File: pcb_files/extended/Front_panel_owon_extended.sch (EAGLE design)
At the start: 17 parts, among them M1 ARDUINO-NANO-3.0, SW1 ROTARTY_ENCODER, SW2 TACTILE-SWITCH-PTH, SW3 TACTILE-SWITCH-PTH, SW4 TACTILE-SWITCH-PTH

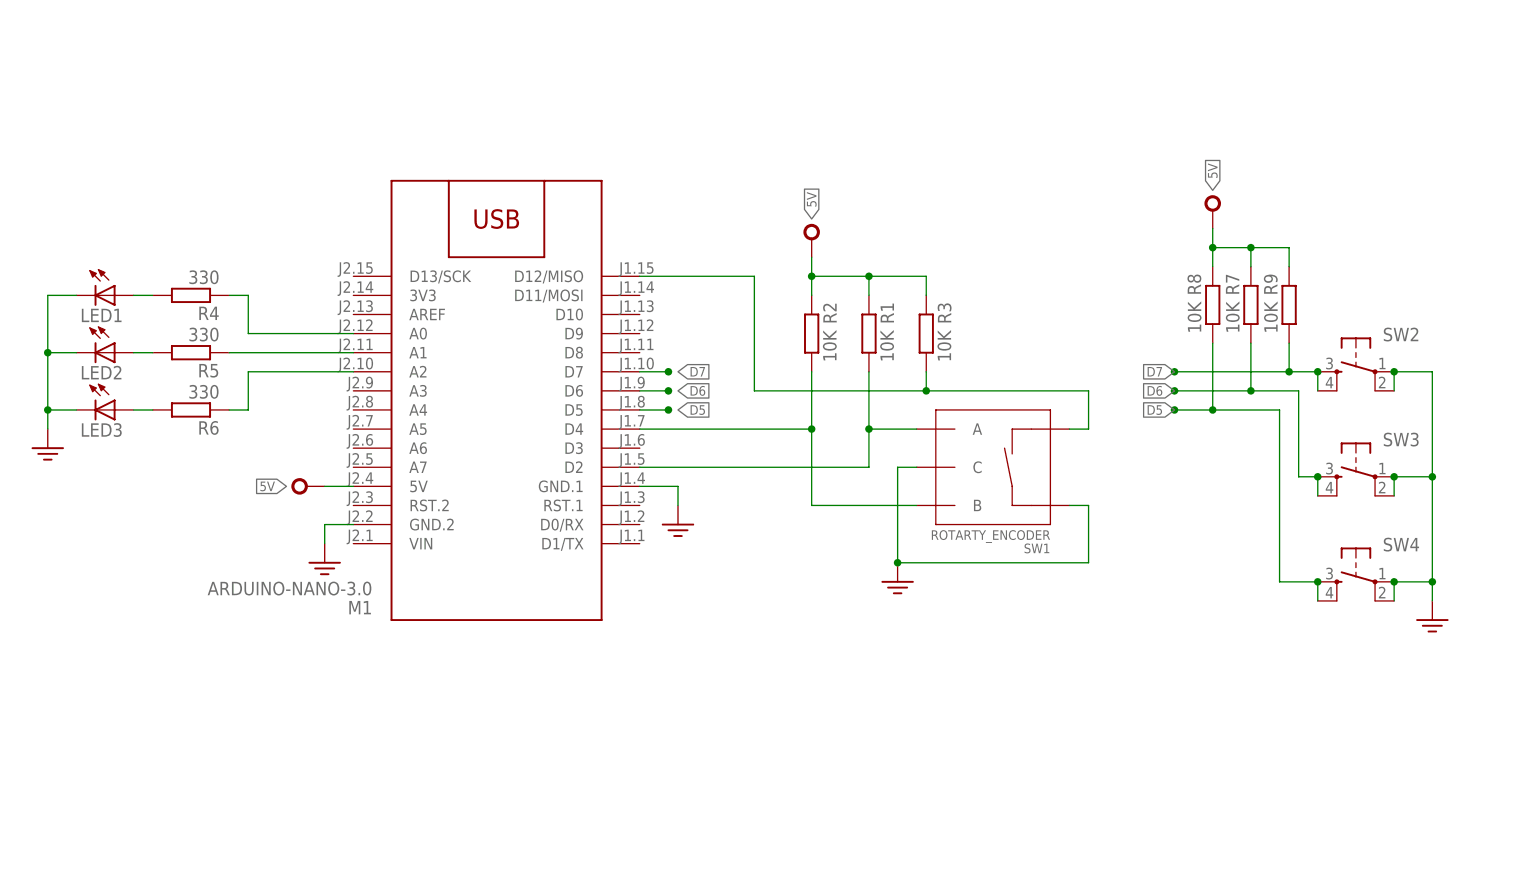
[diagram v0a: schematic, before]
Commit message: retoques, mejoras y agregados
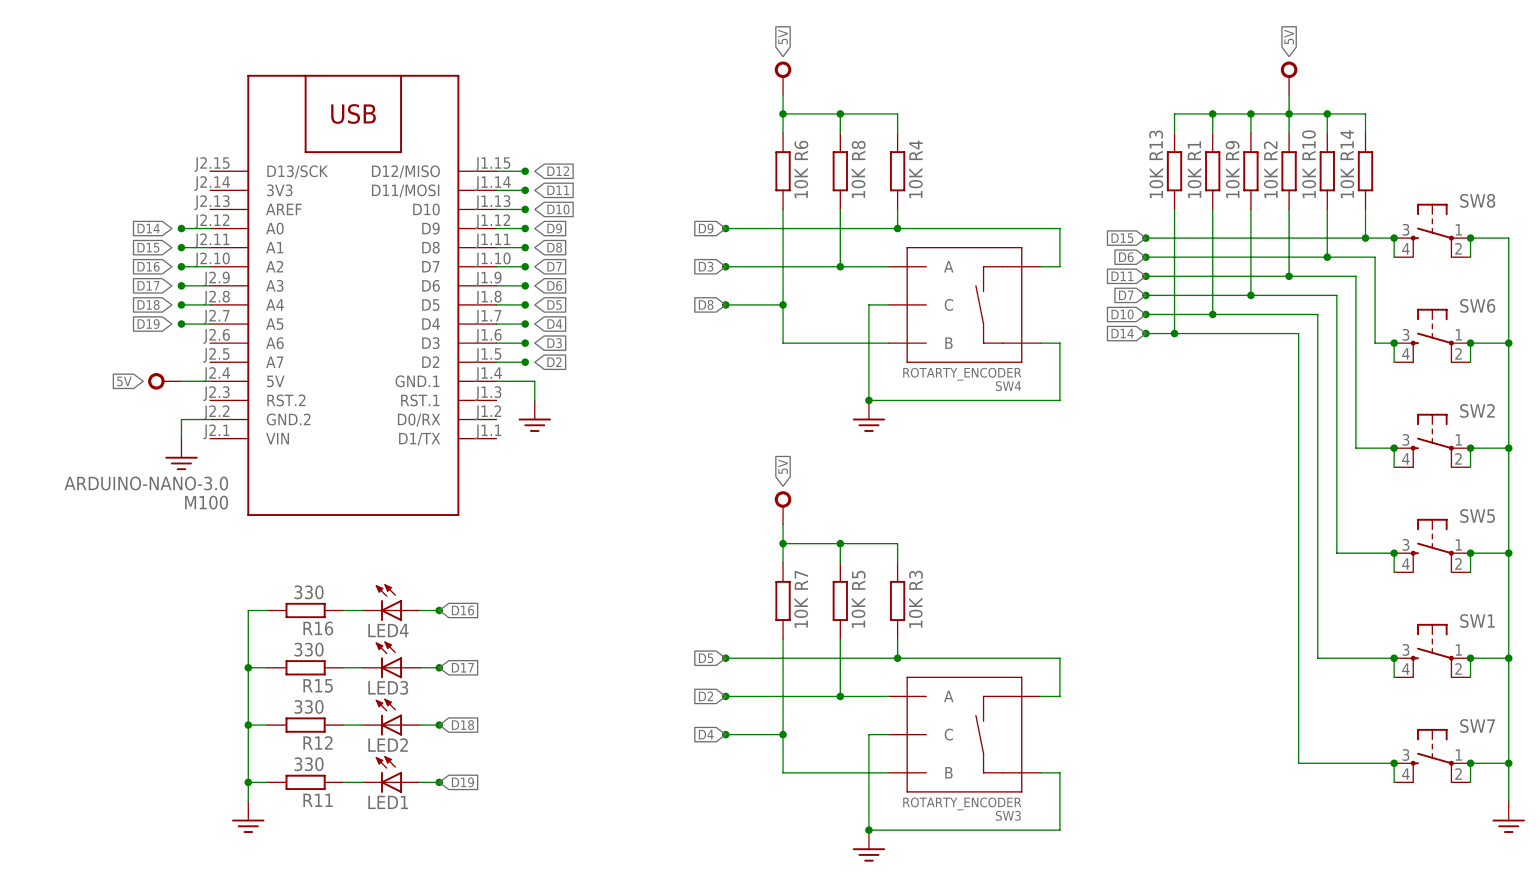
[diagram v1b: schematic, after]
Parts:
- removed M1: ARDUINO-NANO-3.0, diy-modules:ARDUINO-NANO-3.0
- added LED4: (no value), adafruit:LED5MM
- added M100: ARDUINO-NANO-3.0, diy-modules:ARDUINO-NANO-3.0
- added R10, R13, R14: 10K, rcl:R-EU_0204/7
- added R11, R12, R15, R16: 330, rcl:R-EU_0204/7
- added SW5, SW6, SW7, SW8: TACTILE-SWITCH-PTH, GeekAmmo:TACTILE-SWITCH-PTH
- R4, R5, R6: value 330 -> 10K
- SW1: value ROTARTY_ENCODER -> TACTILE-SWITCH-PTH; device SparkFun-Electromechanical:ROTARTY_ENCODER -> GeekAmmo:TACTILE-SWITCH-PTH
- SW3, SW4: value TACTILE-SWITCH-PTH -> ROTARTY_ENCODER; device GeekAmmo:TACTILE-SWITCH-PTH -> SparkFun-Electromechanical:ROTARTY_ENCODER
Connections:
- removed net N$5: M1.A0, R4.1
- removed net N$6: M1.A2, R6.1
- new net D10: M100.D10, R1.1, SW1.3, SW1.4
- new net D11: M100.D11/MOSI, R2.1, SW2.3, SW2.4
- new net D14: M100.A0, R13.1, SW7.3, SW7.4
- new net D15: M100.A1, R14.1, SW8.3, SW8.4
- new net D16: LED4.A, M100.A2
- new net D17: LED3.A, M100.A3
- new net D18: LED2.A, M100.A4
- new net D19: LED1.A, M100.A5
- new net D3: M100.D3, R8.1, SW4.A
- new net D8: M100.D8, R6.1, SW4.B
- new net D9: M100.D9, R4.1, SW4.SW-
- net 5V: now also M100.5V, R10.2, R13.2, R14.2, R4.2, R5.2, R6.2; no longer M1.5V
- net D12: now also M100.D12/MISO; no longer M1.D12/MISO, R3.1, SW1.SW-
- net D2: now also M100.D2, R5.1, SW3.A; no longer M1.D2, R1.1, SW1.A
- net D4: now also M100.D4, R7.1, SW3.B; no longer M1.D4, R2.1, SW1.B
- net D5: now also M100.D5, R3.1, SW3.SW-; no longer M1.D5, R8.1, SW4.3, SW4.4
- net D6: now also M100.D6, R10.1, SW6.3, SW6.4; no longer M1.D6, R7.1, SW3.3, SW3.4
- net D7: now also M100.D7, SW5.3, SW5.4; no longer M1.D7, SW2.3, SW2.4
- net GND: now also M100.GND.1, M100.GND.2, R11.2, R12.2, R15.2, R16.2, SW1.1, SW1.2, SW3.C, SW3.SW+, SW4.C, SW4.SW+, SW5.1, SW5.2, SW6.1, SW6.2, SW7.1, SW7.2, SW8.1, SW8.2; no longer LED1.C, LED2.C, LED3.C, M1.GND.1, M1.GND.2, SW1.C, SW1.SW+, SW3.1, SW3.2, SW4.1, SW4.2
- net N$1: now also LED1.C, R11.1; no longer M1.A1, R5.1
- net N$2: now also LED2.C, R12.1; no longer LED1.A, R4.2
- net N$3: now also LED3.C, R15.1; no longer LED2.A, R5.2
- net N$4: now also LED4.C, R16.1; no longer LED3.A, R6.2
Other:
- moved on the sheet: LED1, LED2, LED3, R1, R2, R3, R4, R5, R6, R7, R8, R9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
